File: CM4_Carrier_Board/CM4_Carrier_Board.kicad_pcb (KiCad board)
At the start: 2 copper layers, 22 x 30 mm, 31 parts, among them J1 Barrel_Jack, J2 DF40C-100DP-0.4V_51_, J3 DF40C-100DP-0.4V_51_, J4 Bus_M.2_Socket_M, J5 HDMI_A, J6 Conn_02x20_Odd_Even, J7 USB_A, U1 IP4786CZ32, U2 LM2596S-5, U3 USBLC6-2SC6

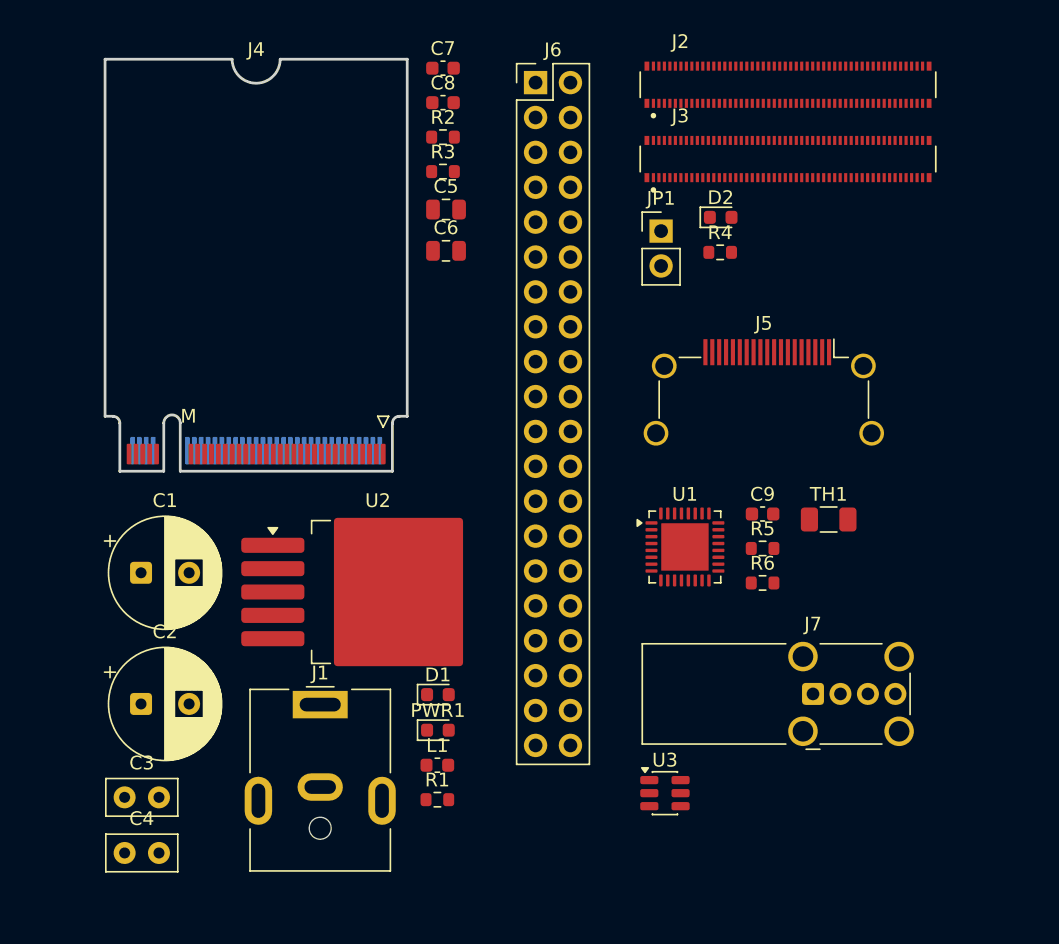
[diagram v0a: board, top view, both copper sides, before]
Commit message: Début de PCB et de routage
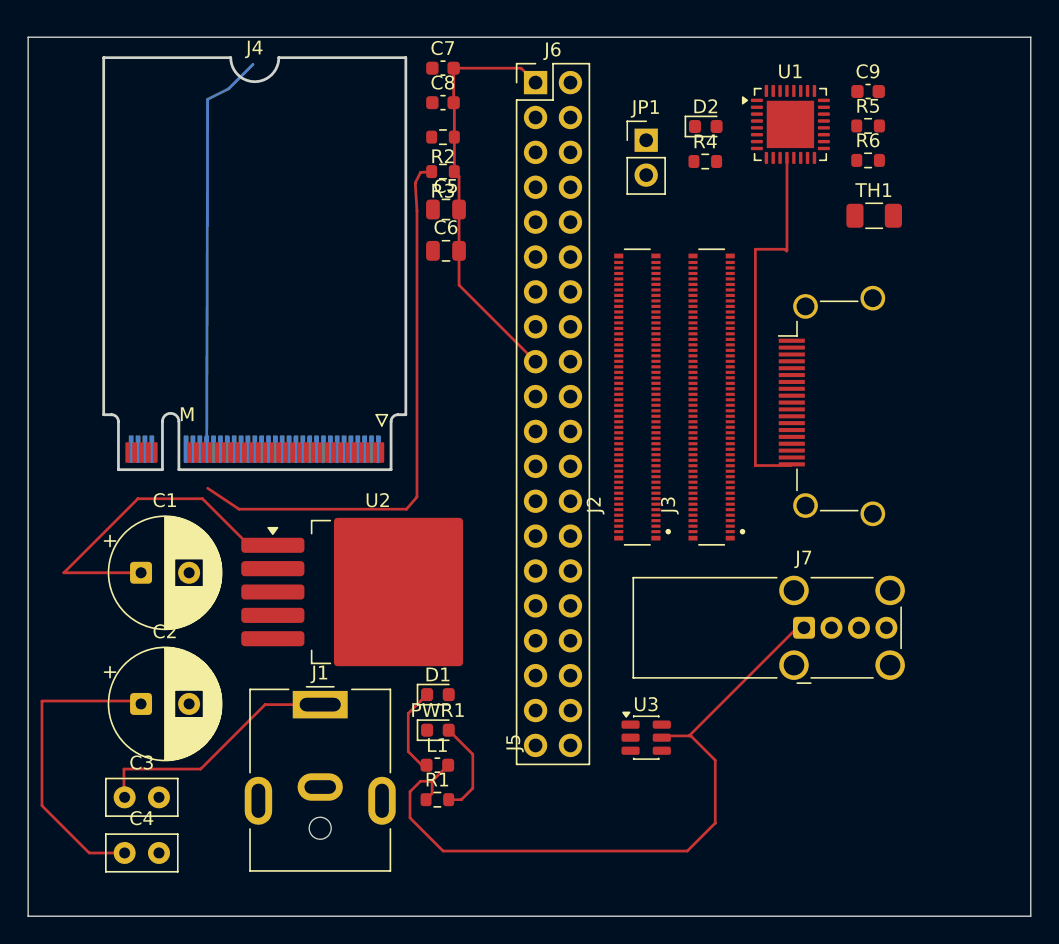
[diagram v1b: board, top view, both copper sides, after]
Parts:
- moved C9 31.7 mm to (108.2, 80.0)
- moved R5 31.7 mm to (108.2, 82.5)
- moved R6 31.7 mm to (108.2, 85.0)
- moved U1 31.7 mm to (102.5, 82.3)
- moved J2 25.2 mm to (91.4, 102.2), turned to 90 degrees
- moved TH1 22.4 mm to (108.6, 89.0)
- moved J3 18.2 mm to (96.8, 102.2), turned to 90 degrees
- moved J5 7.12 mm to (107.6, 102.8), turned to 90 degrees
- moved R4 6.70 mm to (96.3, 85.0)
- moved D2 6.70 mm to (96.3, 82.5)
- moved JP1 6.70 mm to (92.0, 83.5)
- moved J7 4.86 mm to (103.5, 119.0)
- moved U3 4.26 mm to (92.0, 127.0)
- moved J4 0.15 mm to (63.5, 103.5)
- turned R2 to 180 degrees
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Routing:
- net +5V: track 0.00 -> 74.3 mm
- net /Connecteurs/PCIE/PCIe_CLK_nREQ: track 0.00 -> 70.3 mm
- net Net-(U2-VIN): track 0.00 -> 42.8 mm
- net +3.3V: track 0.00 -> 30.2 mm
- net /Connecteurs/Bloc HDMI/HPD: track 0.00 -> 27.6 mm
- net Net-(PWR1-A): track 0.00 -> 7.05 mm
- net Net-(D1-K): track 0.00 -> 6.46 mm
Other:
- board size 22 x 30 mm -> 73 x 64 mm
